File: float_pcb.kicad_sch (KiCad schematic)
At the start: 46 parts, among them J1 BR Switch, J2 5V, J3 USB_C, J4 Conn_01x02, J5 BR_DEPTH_SENSOR, J6 BR Light, J7 Batt, Q1 AO3400A, SW2 SW_Push, SW3 ENABLE, U3 ESP32-S3-MINI-1U

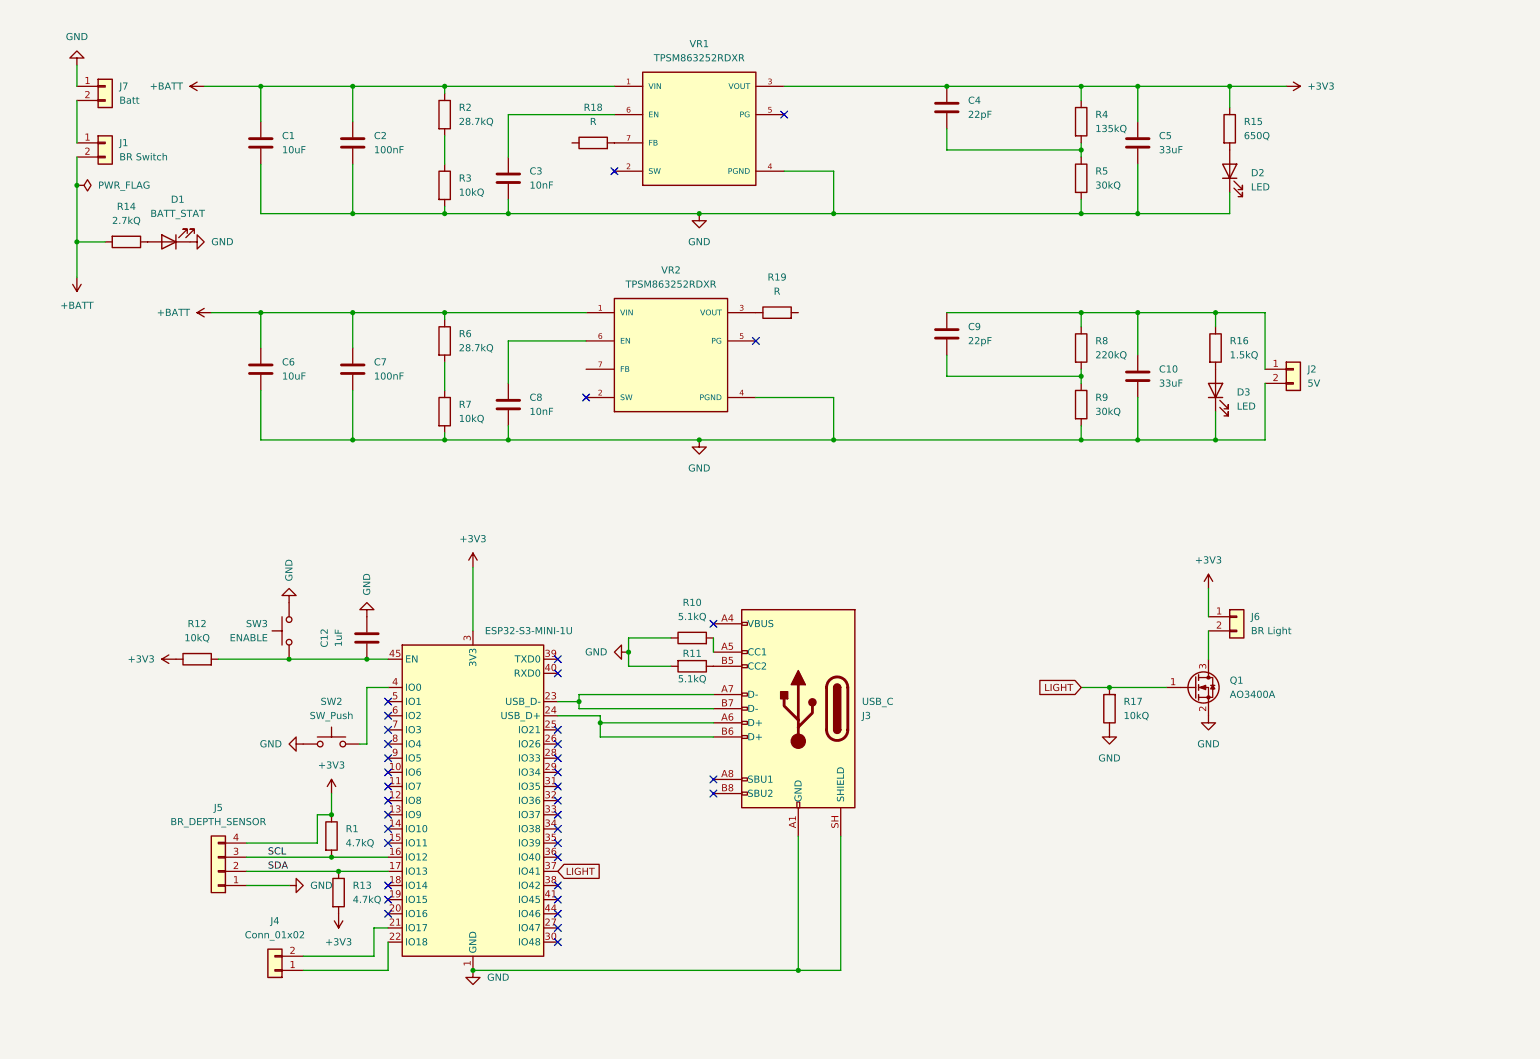
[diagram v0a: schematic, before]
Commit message: First Version
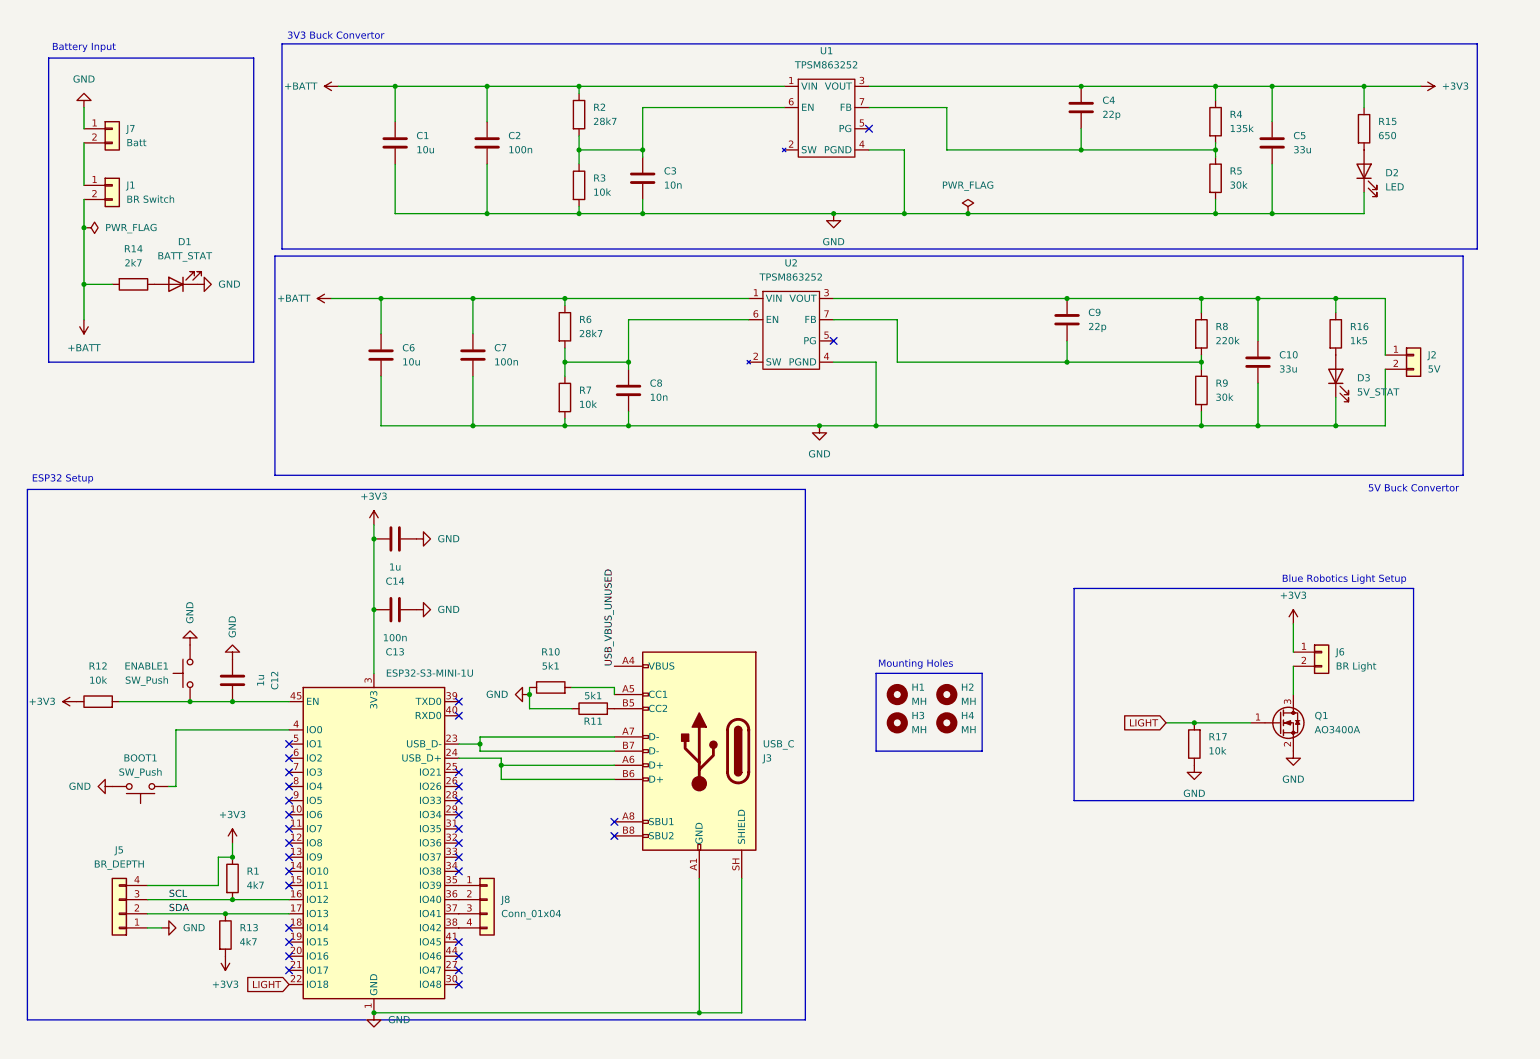
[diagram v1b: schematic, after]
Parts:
- removed J4: Conn_01x02, Connector_PinHeader_2.54mm:PinHeader_1x02_P2.54mm_Vertical, symbol Connector_Generic:Conn_01x02
- removed R18, R19: R, Resistor_SMD:R_0805_2012Metric, symbol Device:R
- removed VR1, VR2: TPSM863252RDXR, TPSM863252RDXR:VREG_TPSM863252RDXR, symbol TPSM863252RDXR:TPSM863252RDXR
- added C13: 100n, Capacitor_SMD:C_0805_2012Metric, symbol Device:C
- added C14: 1u, Capacitor_SMD:C_0805_2012Metric, symbol Device:C
- added H1, H2, H3, H4: MH, MountingHole:MountingHole_2.2mm_M2, symbol Mechanical:MountingHole
- added J8: Conn_01x04, Connector_PinHeader_2.54mm:PinHeader_1x04_P2.54mm_Vertical, symbol Connector_Generic:Conn_01x04
- added U1, U2: TPSM863252, float_pcb_footprints:TPSM86325x_RDX0007A, symbol float_pcb_symbols:TPSM86325X
- C1, C6: value 10uF -> 10u
- C10, C5: value 33uF -> 33u
- C12: value 1uF -> 1u
- C2, C7: value 100nF -> 100n
- C3, C8: value 10nF -> 10n
- C4, C9: value 22pF -> 22p
- D3: value LED -> 5V_STAT
- ENABLE1: renamed from SW3; value ENABLE -> SW_Push
- J1, J2, J6: footprint Connector_JST:JST_VH_B2P-VH_1x02_P3.96mm_Vertical -> Connector_JST:JST_XH_B2B-XH-A_1x02_P2.50mm_Vertical
- J3: footprint Connector_USB:USB_C_Receptacle_HRO_TYPE-C-31-M-12 -> Connector_USB:USB_C_Receptacle_GCT_USB4105-xx-A_16P_TopMnt_Horizontal
- J5: value BR_DEPTH_SENSOR -> BR_DEPTH
- R1, R13: value 4.7kQ -> 4k7
- R10, R11: value 5.1kQ -> 5k1
- R12, R17, R3, R7: value 10kQ -> 10k
- R14: value 2.7kQ -> 2k7
- R15: value 650Q -> 650
- R16: value 1.5kQ -> 1k5; footprint LED_SMD:LED_0805_2012Metric -> Resistor_SMD:R_0805_2012Metric
- R2, R6: value 28.7kQ -> 28k7
- R4: value 135kQ -> 135k
- R5, R9: value 30kQ -> 30k
- R8: value 220kQ -> 220k
- renumbered SW2 to BOOT1
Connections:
- net +3V3: now also C13.1, C14.1, U1.3 (VOUT)
- net +BATT: now also U1.1 (VIN), U2.1 (VIN)
- net GND: now also BOOT1.2, C12.2, R11.1, C13.2, C14.2, U1.4 (PGND), U2.4 (PGND); no longer BOOT1.1, C12.1, R11.2
- net LIGHT: now also U3.22 (IO18); no longer U3.37 (IO41)
- net at C10.1, C9.1, J2.1 (Pin_1)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: now also U2.3 (VOUT)
- net at C9.2, R8.2, R9.1: now also U2.7 (FB)
- net at R6.2, R7.1: now also C8.1, U2.6 (EN)
- net at J3.B5 (CC2): now also R11.2; no longer R11.1
- net at ENABLE1.1, R12.2, U3.45 (EN): now also C12.1; no longer C12.2
- net at C4.2, R4.2, R5.1: now also U1.7 (FB)
- net at U3.4 (IO0): now also BOOT1.1; no longer BOOT1.2
- net USB_VBUS_UNUSED: now reaches J3.A4 (VBUS), J3.A9 (VBUS), J3.B4 (VBUS), J3.B9 (VBUS)
- net at C3.1: now also R2.2, R3.1, U1.6 (EN)
- net at U3.35 (IO39): now also J8.1 (Pin_1)
- net at U3.36 (IO40): now also J8.2 (Pin_2)
- net at U3.38 (IO42): now also J8.4 (Pin_4)
- new net: J8.3 (Pin_3), U3.37 (IO41)
- no-connect marks 38 -> 33
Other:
- note added: "3V3 Buck Convertor"
- note added: "5V Buck Convertor"
- note added: "Battery Input"
- note added: "Blue Robotics Light Setup"
- note added: "ESP32 Setup"
- note added: "Mounting Holes"
- company: (none) -> Leviathan Underwater Robotics (Evan Kim)
- title: (none) -> Float PCB
- moved on the sheet: BOOT1, C1, C10, C12, C2, C3, C4, C5, C6, C7, C8, C9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

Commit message: V2
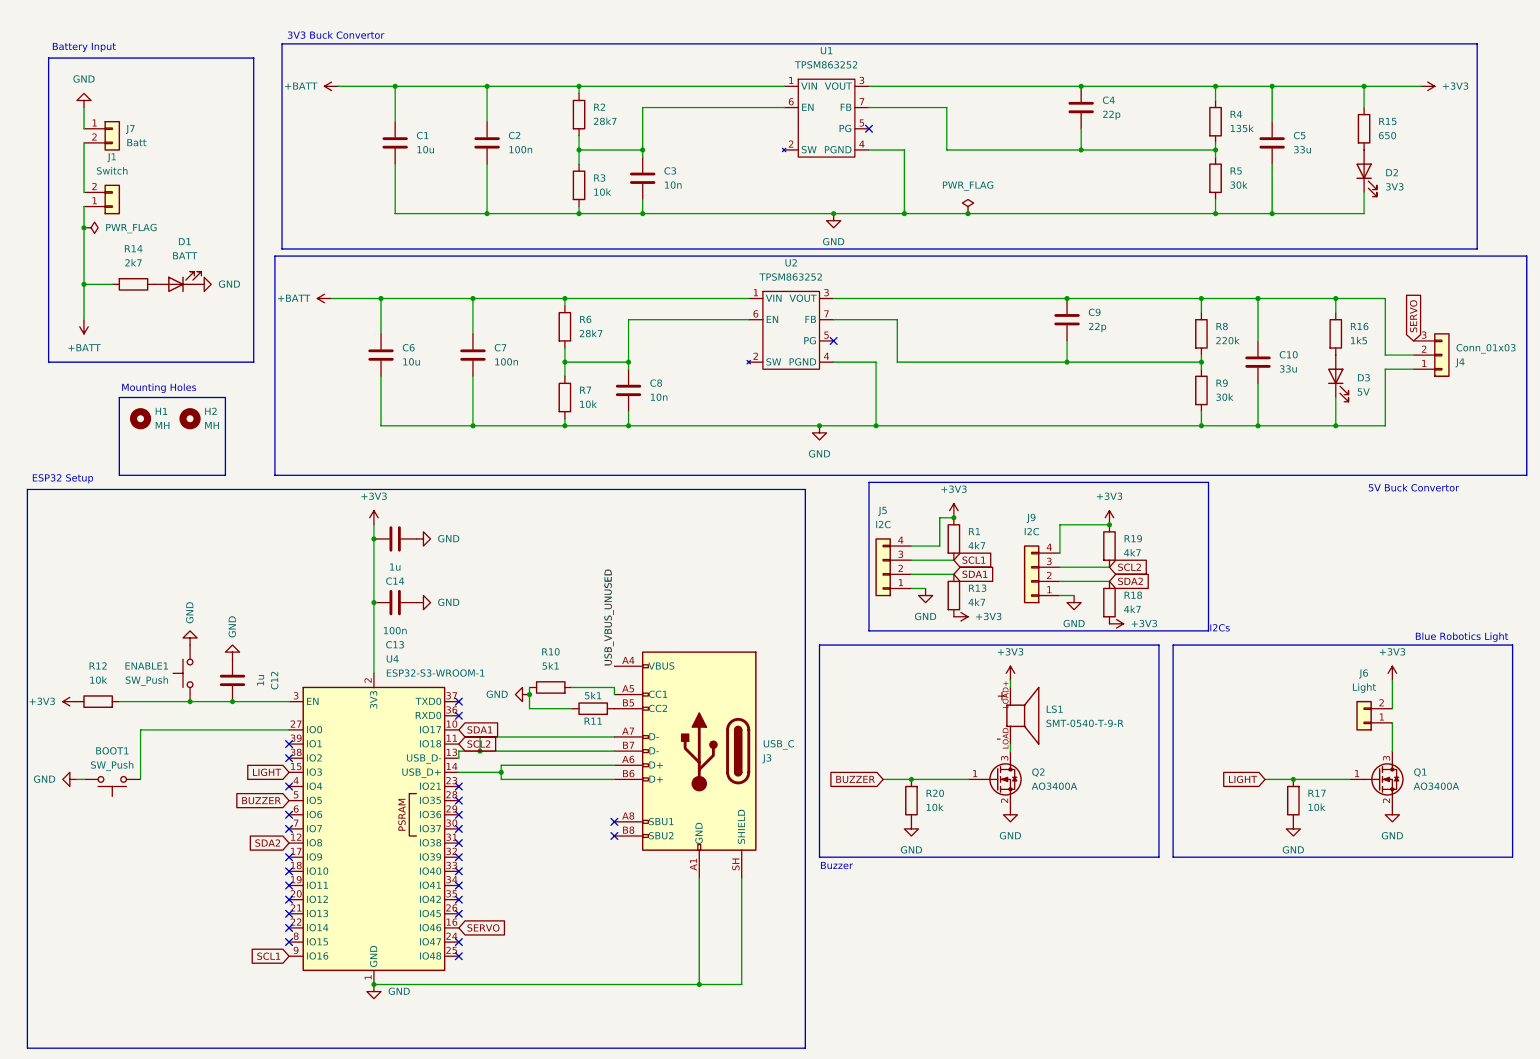
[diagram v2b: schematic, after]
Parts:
- removed H3, H4: MH, MountingHole:MountingHole_2.2mm_M2, symbol Mechanical:MountingHole
- removed J2: 5V, Connector_JST:JST_XH_B2B-XH-A_1x02_P2.50mm_Vertical, symbol Connector_Generic:Conn_01x02
- removed J8: Conn_01x04, Connector_PinHeader_2.54mm:PinHeader_1x04_P2.54mm_Vertical, symbol Connector_Generic:Conn_01x04
- removed U3: ESP32-S3-MINI-1U, RF_Module:ESP32-S2-MINI-1U, symbol RF_Module:ESP32-S3-MINI-1U
- added J4: Conn_01x03, Connector_JST:JST_XH_B3B-XH-A_1x03_P2.50mm_Vertical, symbol Connector_Generic:Conn_01x03
- added J9: I2C, Connector_JST:JST_XH_B4B-XH-A_1x04_P2.50mm_Vertical, symbol Connector_Generic:Conn_01x04
- added LS1: SMT-0540-T-9-R, buzzer:XDCR_SMT-0540-T-9-R, symbol Buzzer:SMT-0540-T-9-R
- added Q2: AO3400A, Package_TO_SOT_SMD:SOT-23, symbol Transistor_FET:AO3400A
- added R18, R19: 4k7, Resistor_SMD:R_0603_1608Metric, symbol Device:R
- added R20: 10k, Resistor_SMD:R_0603_1608Metric, symbol Device:R
- added U4: ESP32-S3-WROOM-1, RF_Module:ESP32-S3-WROOM-1U, symbol RF_Module:ESP32-S3-WROOM-1
- C1, C10, C12, C13, C14, C2, C3, C4, C5, C6, C7, C8, C9: footprint Capacitor_SMD:C_0805_2012Metric -> Capacitor_SMD:C_0603_1608Metric
- D1: value BATT_STAT -> BATT; footprint LED_SMD:LED_0805_2012Metric -> LED_SMD:LED_0603_1608Metric
- D2: value LED -> 3V3; footprint LED_SMD:LED_0805_2012Metric -> LED_SMD:LED_0603_1608Metric
- D3: value 5V_STAT -> 5V; footprint LED_SMD:LED_0805_2012Metric -> LED_SMD:LED_0603_1608Metric
- J1: value BR Switch -> Switch
- J5: value BR_DEPTH -> I2C; footprint Connector_JST:JST_GH_BM04B-GHS-TBT_1x04-1MP_P1.25mm_Vertical -> Connector_JST:JST_XH_B4B-XH-A_1x04_P2.50mm_Vertical
- J6: value BR Light -> Light
- R1, R10, R11, R12, R13, R14, R15, R16, R17, R2, R3, R4, R5, R6, R7, R8, R9: footprint Resistor_SMD:R_0805_2012Metric -> Resistor_SMD:R_0603_1608Metric
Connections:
- net +3V3: now also J6.2 (Pin_2), J9.4 (Pin_4), LS1.LOAD+, R18.2, R19.1, U4.2 (3V3); no longer J6.1 (Pin_1)
- net +BATT: now also C1.2, C7.2, J1.1 (Pin_1); no longer C1.1, C7.1, J1.2 (Pin_2)
- net GND: now also C1.1, C7.1, J4.1 (Pin_1), J9.1 (Pin_1), Q2.2 (S), R20.1, U4.1 (GND), U4.40 (GND), U4.41 (GND); no longer C1.2, C7.2
- net LIGHT: now also U4.15 (IO3)
- net at C10.1, C9.1, R16.1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: now also J4.2 (Pin_2)
- net at C12.1, ENABLE1.1, R12.2: now also U4.3 (EN)
- net at J7.2 (Pin_2): now also J1.2 (Pin_2); no longer J1.1 (Pin_1)
- net at BOOT1.1: now also U4.27 (IO0)
- net at J3.A6 (D+), J3.B6 (D+): now also U4.14 (USB_D+)
- net at J3.A7 (D-), J3.B7 (D-): now also U4.13 (USB_D-)
- net at Q1.3 (D): now also J6.1 (Pin_1); no longer J6.2 (Pin_2)
- net SCL renamed SCL1
- net SCL1: now also U4.9 (IO16)
- net SDA renamed SDA1
- net SDA1: now also U4.10 (IO17)
- new net: LS1.LOAD-, Q2.3 (D)
- new net BUZZER: Q2.1 (G), R20.2, U4.5 (IO5)
- new net SCL2: J9.3 (Pin_3), R19.2, U4.11 (IO18)
- new net SDA2: J9.2 (Pin_2), R18.1, U4.12 (IO8)
- new net SERVO: J4.3 (Pin_3), U4.16 (IO46)
- no-connect marks 33 -> 30
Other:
- note added: "Blue Robotics Light"
- note added: "Buzzer"
- note added: "I2Cs"
- note removed: "Blue Robotics Light Setup"
- title: Float PCB -> Dory
- moved on the sheet: BOOT1, C1, C13, C7, H1, H2, J1, J6, Q1, R17

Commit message: V3
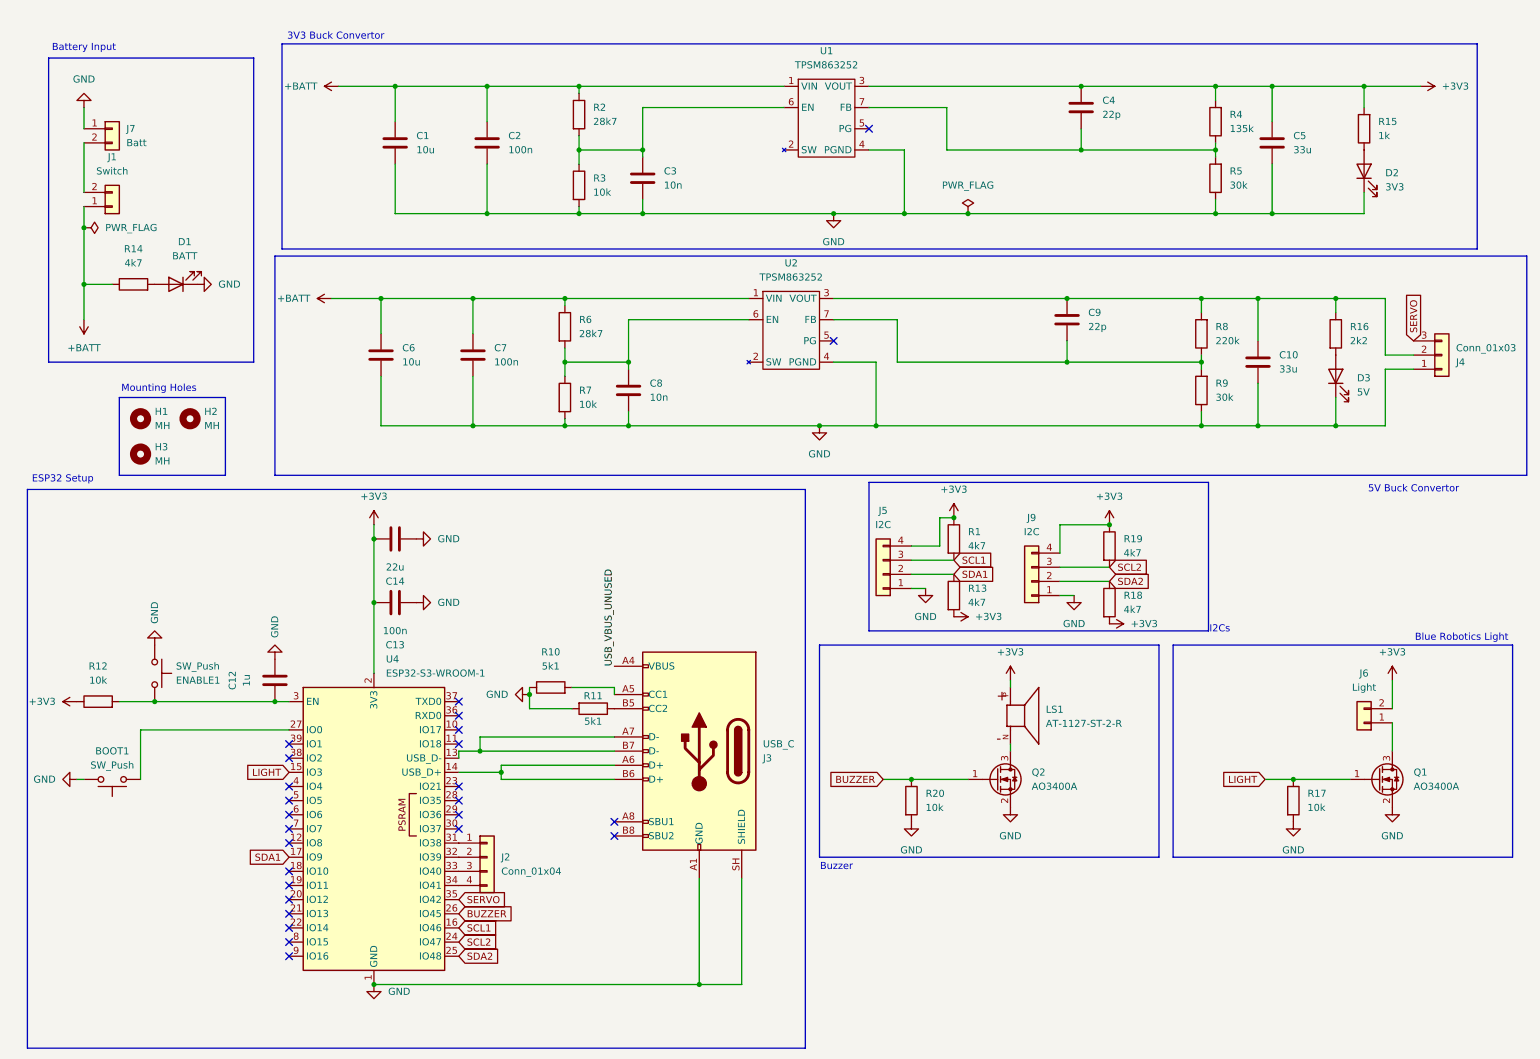
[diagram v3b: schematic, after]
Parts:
- removed LS1: SMT-0540-T-9-R, buzzer:XDCR_SMT-0540-T-9-R, symbol Buzzer:SMT-0540-T-9-R
- added H3: MH, MountingHole:MountingHole_2.2mm_M2, symbol Mechanical:MountingHole
- added J2: Conn_01x04, Connector_PinHeader_2.54mm:PinHeader_1x04_P2.54mm_Vertical, symbol Connector_Generic:Conn_01x04
- added LS1: AT-1127-ST-2-R, buzzer:XDCR_AT-1127-ST-2-R, symbol Buzzer:AT-1127-ST-2-R
- C14: value 1u -> 22u
- R14: value 2k7 -> 4k7
- R15: value 650 -> 1k
- R16: value 1k5 -> 2k2
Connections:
- net +3V3: now also C4.2, C5.2, R15.2, R4.2, LS1.P; no longer C4.1, C5.1, R15.1, R4.1
- net +BATT: now also R14.1; no longer R14.2
- net BUZZER: now also R20.1, U4.26 (IO45); no longer R20.2, U4.5 (IO5)
- net GND: now also C10.1, C12.1, C5.1, ENABLE1.1, R11.2, R17.2, R20.2, R5.1, R9.1; no longer C10.2, C12.2, C5.2, ENABLE1.2, R11.1, R17.1, R20.1, R5.2, R9.2
- net LIGHT: now also R17.1; no longer R17.2
- net SCL1: now also U4.16 (IO46); no longer U4.9 (IO16)
- net SCL2: now also U4.24 (IO47); no longer U4.11 (IO18)
- net SDA1: now also U4.17 (IO9); no longer U4.10 (IO17)
- net SDA2: now also U4.25 (IO48); no longer U4.12 (IO8)
- net SERVO: now also U4.35 (IO42); no longer U4.16 (IO46)
- net at J4.2 (Pin_2), R16.1, U2.3 (VOUT): now also C10.2, C9.2, R8.2; no longer C10.1, C9.1, R8.1
- net at J3.B5 (CC2): now also R11.1; no longer R11.2
- net at Q2.3 (D): now also LS1.N
- net at R12.2, U4.3 (EN): now also C12.2, ENABLE1.2; no longer C12.1, ENABLE1.1
- net at U4.31 (IO38): now also J2.1 (Pin_1)
- net at U4.32 (IO39): now also J2.2 (Pin_2)
- net at U4.33 (IO40): now also J2.3 (Pin_3)
- net at U4.34 (IO41): now also J2.4 (Pin_4)
- net at D2.2 (A): now also R15.1; no longer R15.2
- net at D1.2 (A): now also R14.2; no longer R14.1
- new net: C9.1, R8.1, R9.2, U2.7 (FB)
- new net: C4.1, R4.1, R5.2, U1.7 (FB)
- no-connect marks 30 -> 26
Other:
- company: Leviathan Underwater Robotics (Evan Kim) -> Leviathan Underwater Robotics
- moved on the sheet: C10, C12, C4, C5, C9, ENABLE1, R11, R14, R15, R17, R20, R4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
